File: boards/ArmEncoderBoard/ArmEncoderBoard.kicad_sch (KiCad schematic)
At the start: 25 parts, among them J1 Conn_01x05, Q1 SS8050, Q2 SS8050, U1 SN74LVC2G17DBVR, U2 AS5045B

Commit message: Order arm encoder board, update bom
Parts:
- D1: footprint LedBlue:YLED0603B -> LedBlue:150080BS75000_Modified; LCSC C19171394 -> C6067133
- D2: footprint LedRed:YLED0603R -> LedRed:NCD0603R1; LCSC C19171390 -> C84263
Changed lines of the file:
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@@
 			)
 		)
-		(property "Footprint" "LedRed:YLED0603R"
+		(property "Footprint" "LedRed:NCD0603R1"
 			(at 176.53 139.7 0)
 			(effects
@@
 			)
 		)
-		(property "LCSC" "C19171390"
+		(property "LCSC" "C84263"
 			(at 174.9425 133.35 0)
 			(effects
@@
 			)
 		)
-		(property "Footprint" "LedBlue:YLED0603B"
+		(property "Footprint" "LedBlue:150080BS75000_Modified"
 			(at 176.53 116.84 0)
 			(effects
@@
 			)
 		)
-		(property "LCSC" "C19171394"
+		(property "LCSC" "C6067133"
 			(at 174.9425 110.49 0)
 			(effects

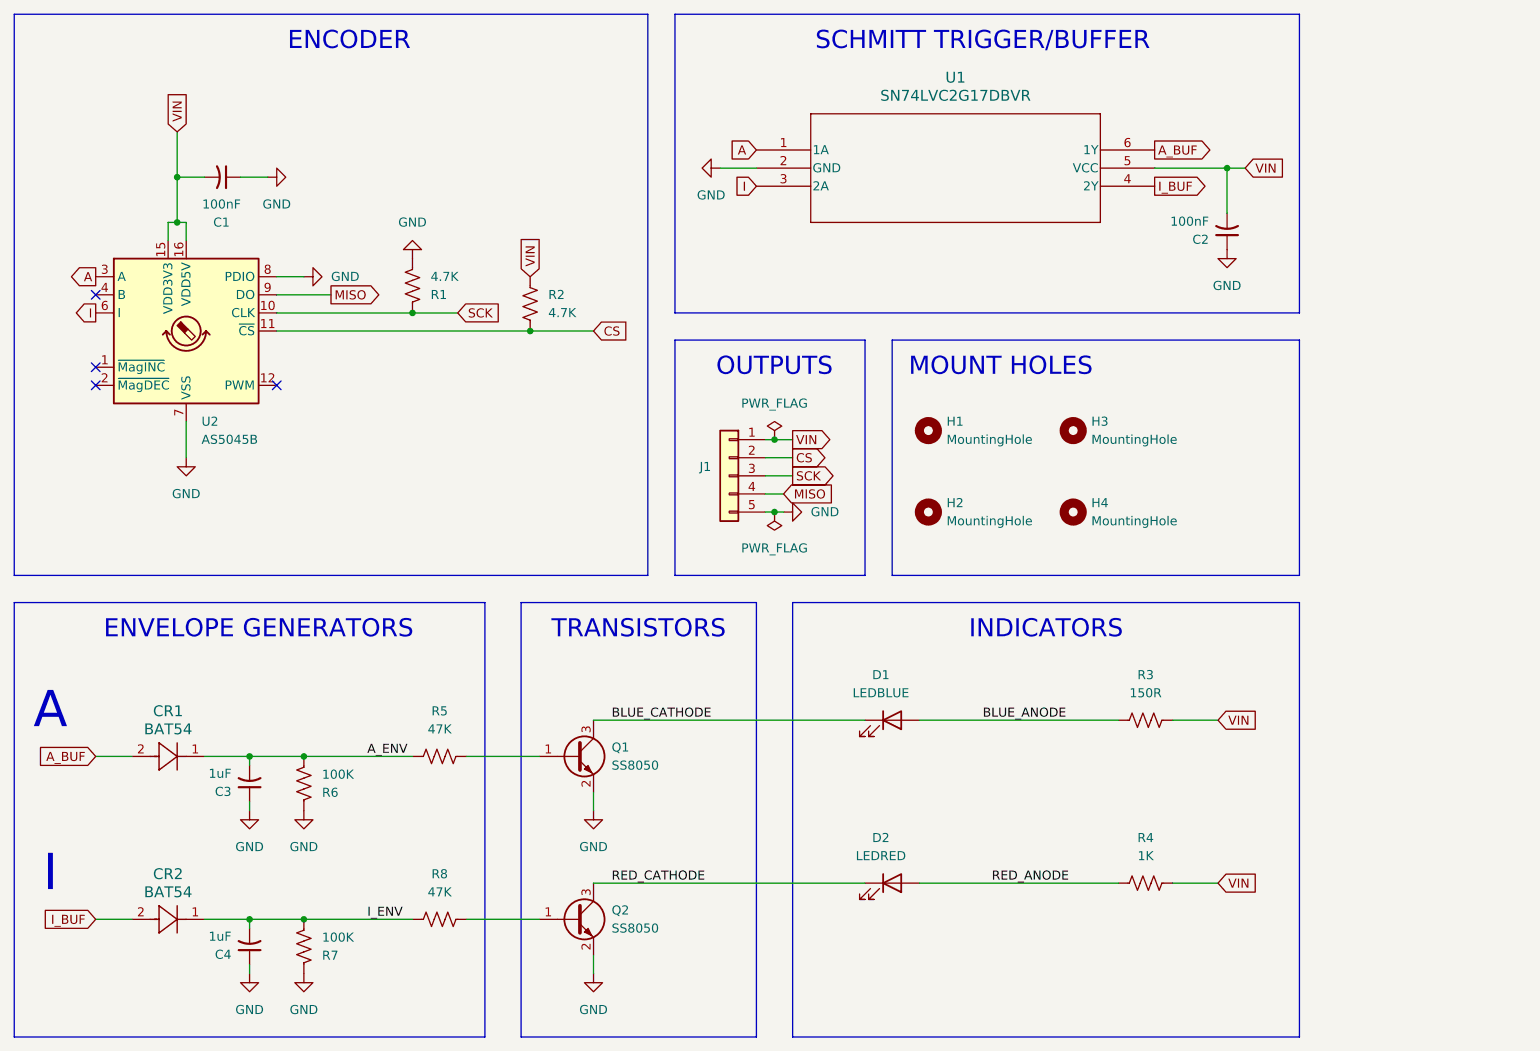
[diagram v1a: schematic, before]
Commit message: Update main and leg board
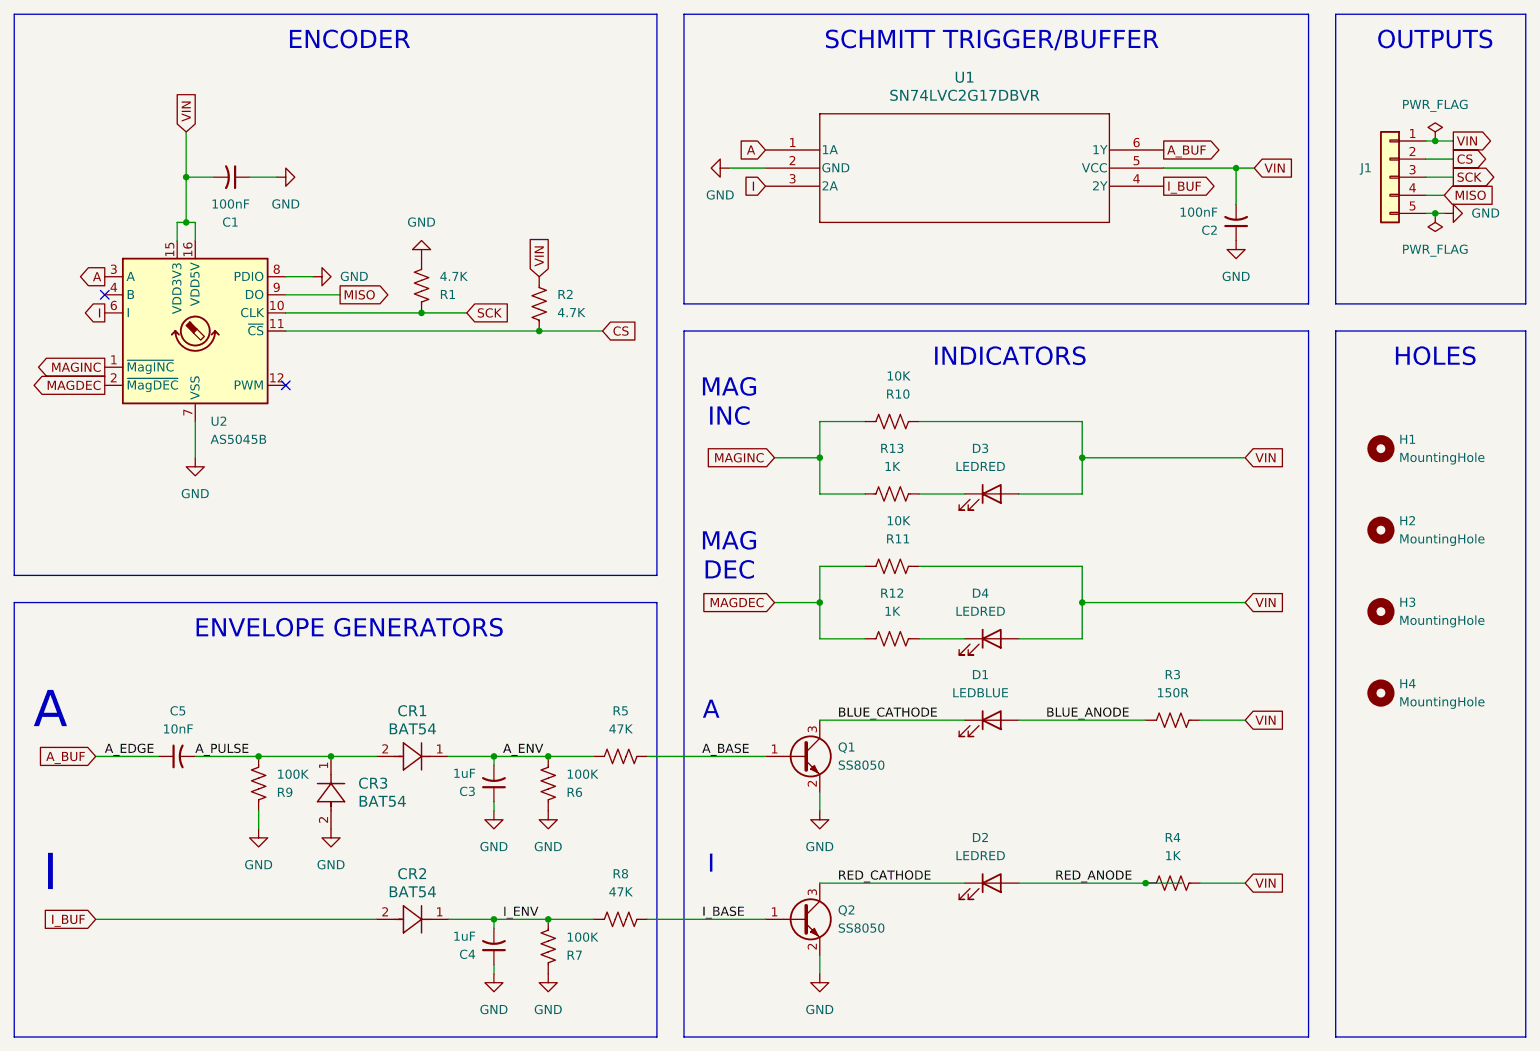
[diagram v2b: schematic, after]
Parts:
- added C5: 10nF, Capacitor10nF:GRM1885C1H103JA01D, symbol Device:C_Small_US
- added CR3: BAT54, EnvelopeDiode:BAT54WS-7-F, symbol EnvelopeDiode:BAT54WS-7-F
- added D3, D4: LEDRED, LedRed:NCD0603R1, symbol Device:LED
- added R10, R11: 10K, Resistor10K:CRCW060310K0FKEA, symbol Device:R_US
- added R12, R13: 1K, Resistor1K:RCG06031K00FKEA, symbol Device:R_US
- added R9: 100K, Resistor100K:CRCW0603100KFKEA, symbol Device:R_US
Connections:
- net A_BUF: now also C5.1; no longer CR1.2
- net GND: now also CR3.2, R9.1
- net VIN: now also D3.2 (A), D4.2 (A), R10.1, R11.1
- net I_BASE: now reaches Q2.1 (B), R8.1
- net MAGINC: now reaches U2.1 (~{MagINC})
- net MAGINC: now also R10.2, R13.2
- net MAGDEC: now reaches U2.2 (~{MagDEC})
- net MAGDEC: now also R11.2, R12.2
- net A_BASE: now reaches Q1.1 (B), R5.1
- new net: D3.1 (K), R13.1
- new net: D4.1 (K), R12.1
- new net A_PULSE: C5.2, CR1.2, CR3.1, R9.2
- no-connect marks 4 -> 2
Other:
- note added: "HOLES"
- note added: "MAG DEC"
- note added: "MAG INC"
- note removed: "MOUNT HOLES"
- note removed: "TRANSISTORS"
- moved on the sheet: C1, C2, C3, C4, CR1, CR2, D1, D2, H1, H2, H3, H4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
